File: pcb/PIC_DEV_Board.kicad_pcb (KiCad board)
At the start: 4 copper layers, 51 x 32 mm, 31 parts, among them J1 Conn_01x08_Pin, J3 Conn_01x02_Pin, J4 Conn_01x02_Pin, J5 Conn_01x01_Pin, U3 MCP3002, U4 MCP4801, U5 FT230XS

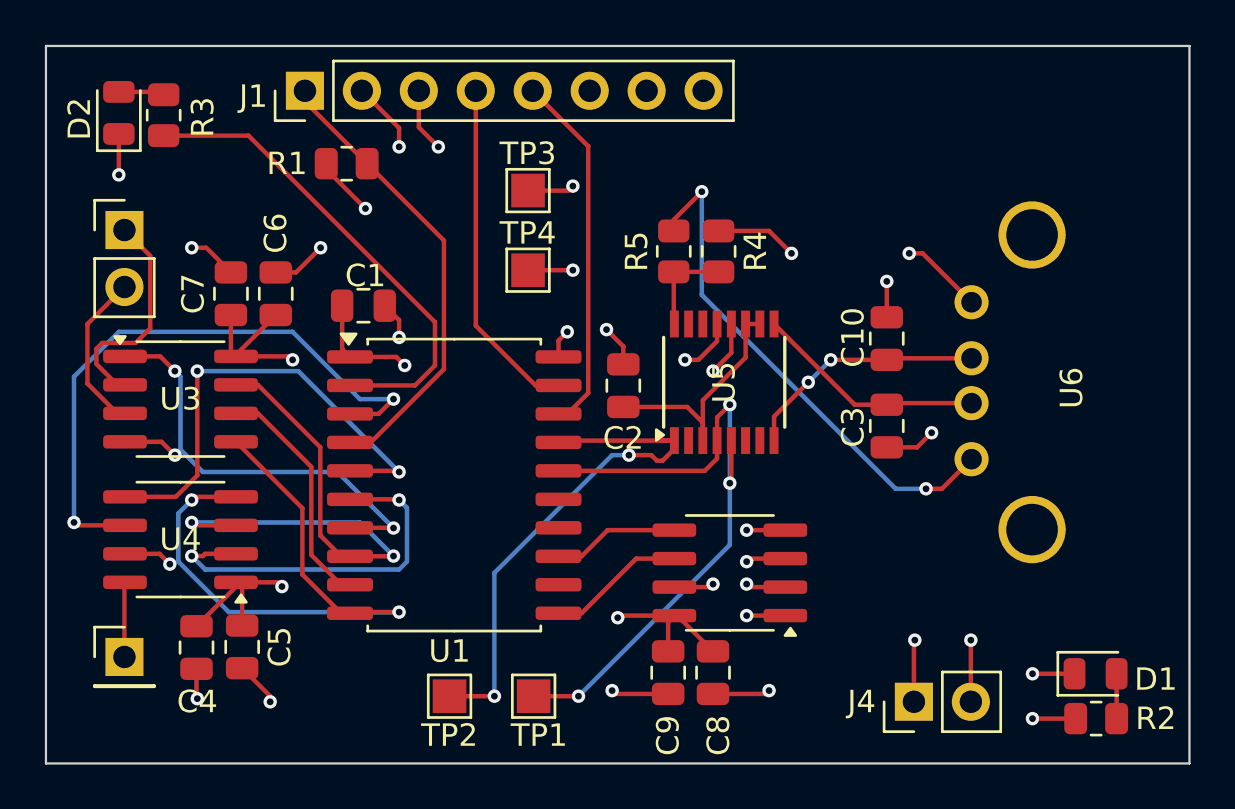
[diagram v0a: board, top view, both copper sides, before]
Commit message: Rev02 final
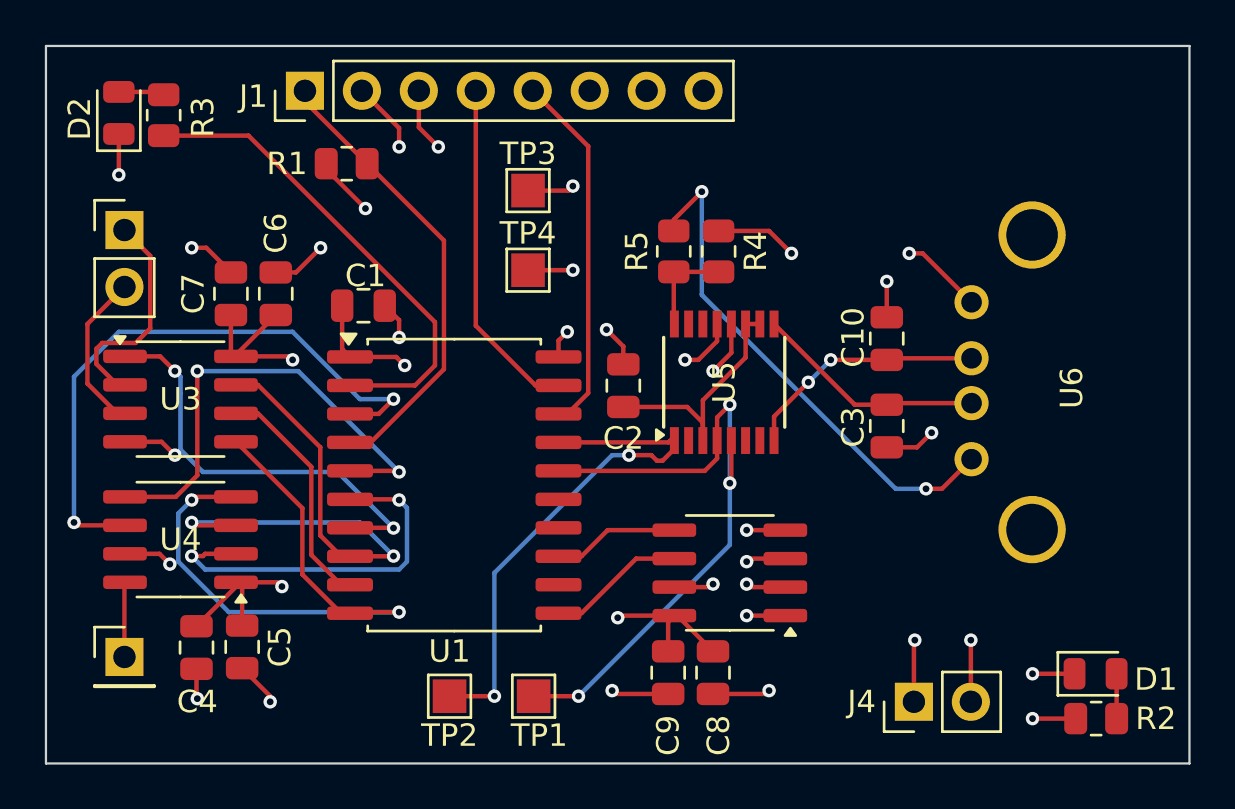
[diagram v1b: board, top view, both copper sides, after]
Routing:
- net Net-(U1-RA2): track 24.2 -> 23.7 mm
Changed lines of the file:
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@@
 			)
 		)
-		(property ki_fp_filters "R_*")
-		(sheetname "Root")
-		(sheetfile "PIC_DEV_Board.kicad_sch")
 		(attr smd)
 		(fp_line
@@
 			(size 1.025 1.4)
 			(layers "F.Cu" "F.Paste" "F.Mask")
-			(roundrect_rratio 0.243902)
+			(roundrect_rratio 0.243902439)
 			(net 7 "Earth")
 			(pintype "passive")
@@
 			(size 1.025 1.4)
 			(layers "F.Cu" "F.Paste" "F.Mask")
-			(roundrect_rratio 0.243902)
+			(roundrect_rratio 0.243902439)
 			(net 36 "/VBUS_SENSE")
 			(pintype "passive")
@@
 			)
 		)
-		(property ki_fp_filters "R_*")
-		(sheetname "Root")
-		(sheetfile "PIC_DEV_Board.kicad_sch")
 		(attr smd)
 		(fp_line
@@
 			(size 1.025 1.4)
 			(layers "F.Cu" "F.Paste" "F.Mask")
-			(roundrect_rratio 0.243902)
+			(roundrect_rratio 0.243902439)
 			(net 8 "+3V3")
 			(pintype "passive")
@@
 			(size 1.025 1.4)
 			(layers "F.Cu" "F.Paste" "F.Mask")
-			(roundrect_rratio 0.243902)
+			(roundrect_rratio 0.243902439)
 			(net 1 "Net-(D1-A)")
 			(pintype "passive")
@@
 			)
 		)
-		(property ki_fp_filters "R_*")
-		(sheetname "Root")
-		(sheetfile "PIC_DEV_Board.kicad_sch")
 		(attr smd)
 		(fp_line
@@
 			(size 1.025 1.4)
 			(layers "F.Cu" "F.Paste" "F.Mask")
-			(roundrect_rratio 0.243902)
+			(roundrect_rratio 0.243902439)
 			(net 32 "Net-(U1-RA5)")
 			(pintype "passive")
@@
 			(size 1.025 1.4)
 			(layers "F.Cu" "F.Paste" "F.Mask")
-			(roundrect_rratio 0.243902)
+			(roundrect_rratio 0.243902439)
 			(net 31 "Net-(D2-A)")
 			(pintype "passive")
@@
 			)
 		)
-		(property ki_fp_filters "R_*")
-		(sheetname "Root")
-		(sheetfile "PIC_DEV_Board.kicad_sch")
 		(attr smd)
 		(fp_line
@@
 			(size 1.025 1.4)
 			(layers "F.Cu" "F.Paste" "F.Mask")
-			(roundrect_rratio 0.243902)
+			(roundrect_rratio 0.243902439)
 			(net 8 "+3V3")
 			(pintype "passive")
@@
 			(size 1.025 1.4)
 			(layers "F.Cu" "F.Paste" "F.Mask")
-			(roundrect_rratio 0.243902)
+			(roundrect_rratio 0.243902439)
 			(net 25 "/Vpp{slash}RA3{slash}MCLR")
 			(pintype "passive")
@@
 			)
 		)
-		(property ki_fp_filters "R_*")
-		(sheetname "Root")
-		(sheetfile "PIC_DEV_Board.kicad_sch")
 		(attr smd)
 		(fp_line
@@
 			(size 1.025 1.4)
 			(layers "F.Cu" "F.Paste" "F.Mask")
-			(roundrect_rratio 0.243902)
+			(roundrect_rratio 0.243902439)
 			(net 36 "/VBUS_SENSE")
 			(pintype "passive")
@@
 			(size 1.025 1.4)
 			(layers "F.Cu" "F.Paste" "F.Mask")
-			(roundrect_rratio 0.243902)
+			(roundrect_rratio 0.243902439)
 			(net 35 "Net-(U6-VCC)")
 			(pintype "passive")
@@
 	)
 	(segment
-		(start 154.75 100)
-		(end 154.5 99.75)
+		(start 155.35 99.1)
+		(end 155.27 99.18)
 		(width 0.2)
 		(layer "F.Cu")
@@
 	)
 	(segment
-		(start 155.5275 99.1)
-		(end 150.44 99.1)
+		(start 154.75 100)
+		(end 154.5 99.75)
 		(width 0.2)
 		(layer "F.Cu")
@@
 	)
 	(segment
-		(start 154.9 99.1)
-		(end 155.5275 99.1)
+		(start 155.27 99.18)
+		(end 150.36 99.18)
 		(width 0.2)
 		(layer "F.Cu")
@@
 		(width 0.2)
 		(layer "F.Cu")
+		(net 19)
+	)
+	(segment
+		(start 155.5275 99.1)
+		(end 155.35 99.1)
+		(width 0.2)
+		(layer "F.Cu")
